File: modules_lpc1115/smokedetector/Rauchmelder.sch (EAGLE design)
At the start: 75 parts, among them IC100 BD9G101, IC2 LPC1115, Q1 BC856, Q3 BCP52, Q4 ASFL, T1 BC847C, T2 BC817

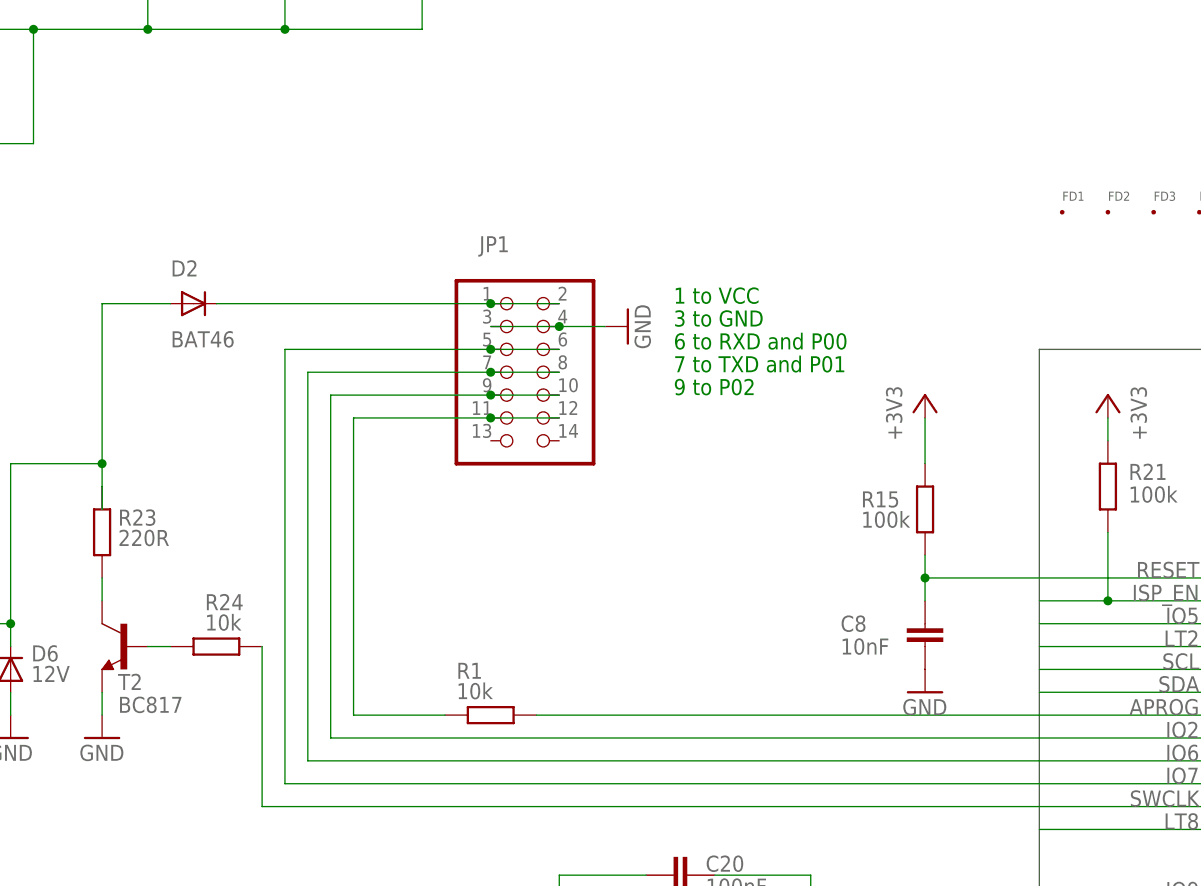
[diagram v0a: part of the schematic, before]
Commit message: [RM] - power feedback protection added
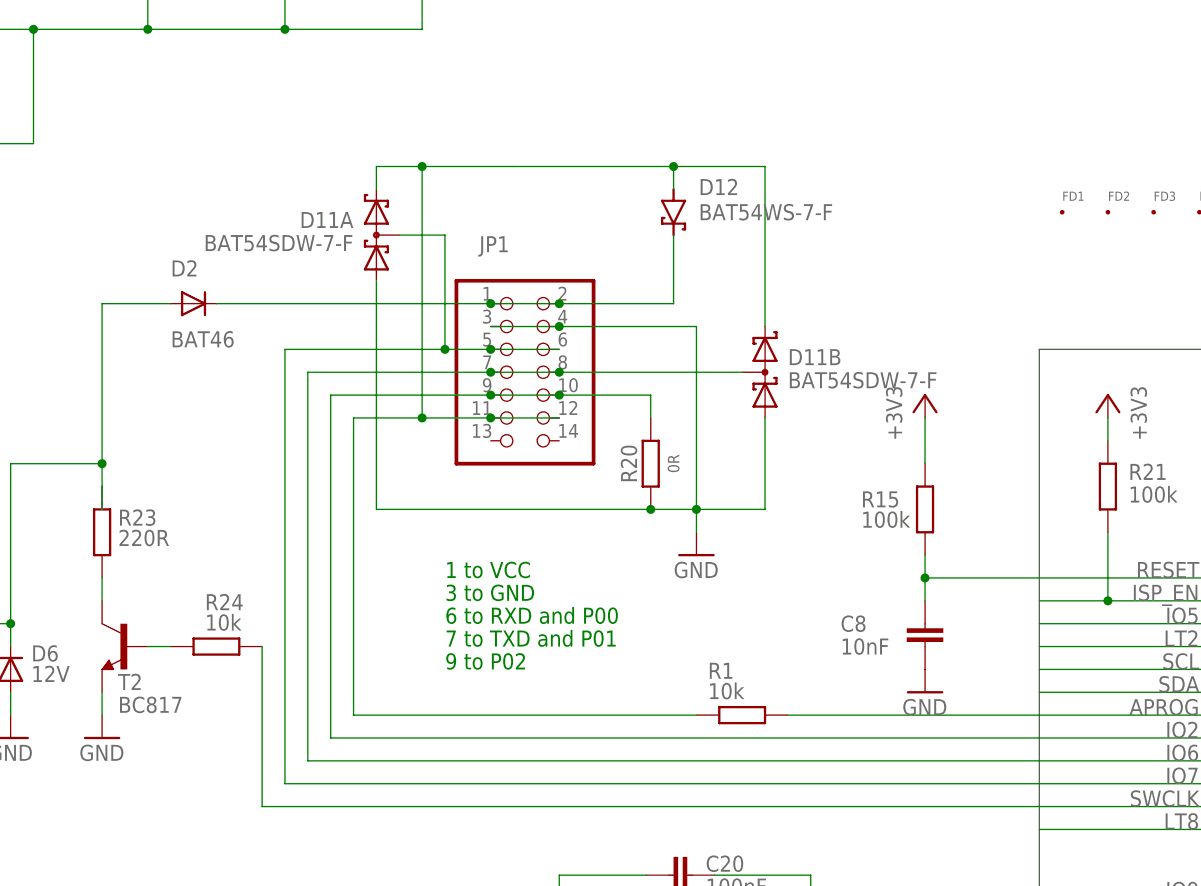
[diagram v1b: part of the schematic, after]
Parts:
- added D11: BAT54SDW-7-F, MyDiode:BAT54SDW-7-F
- added D12: BAT54WS-7-F, MyDiode:BAT54WS-7-F
- added R20: 0R, MyRCL:R-EU_R0805
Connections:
- net GND: now also D11A.A, D11B.A, R20.1
- net LT5: now also R20.2
- net N$1: now also D11A.C, D11B.C, D12.A
- net N$18: now also D12.C
- net RXD: now also D11A.AC
- net TXD: now also D11B.AC
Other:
- moved on the sheet: R1
